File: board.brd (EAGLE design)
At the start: 53.3 x 41.9 mm, 6 parts, among them J1 POWER_JACK, J2 POWER_JACK, J3 POWER_JACK, J4 POWER_JACK, J5 POWER_JACK, J6 POWER_JACK

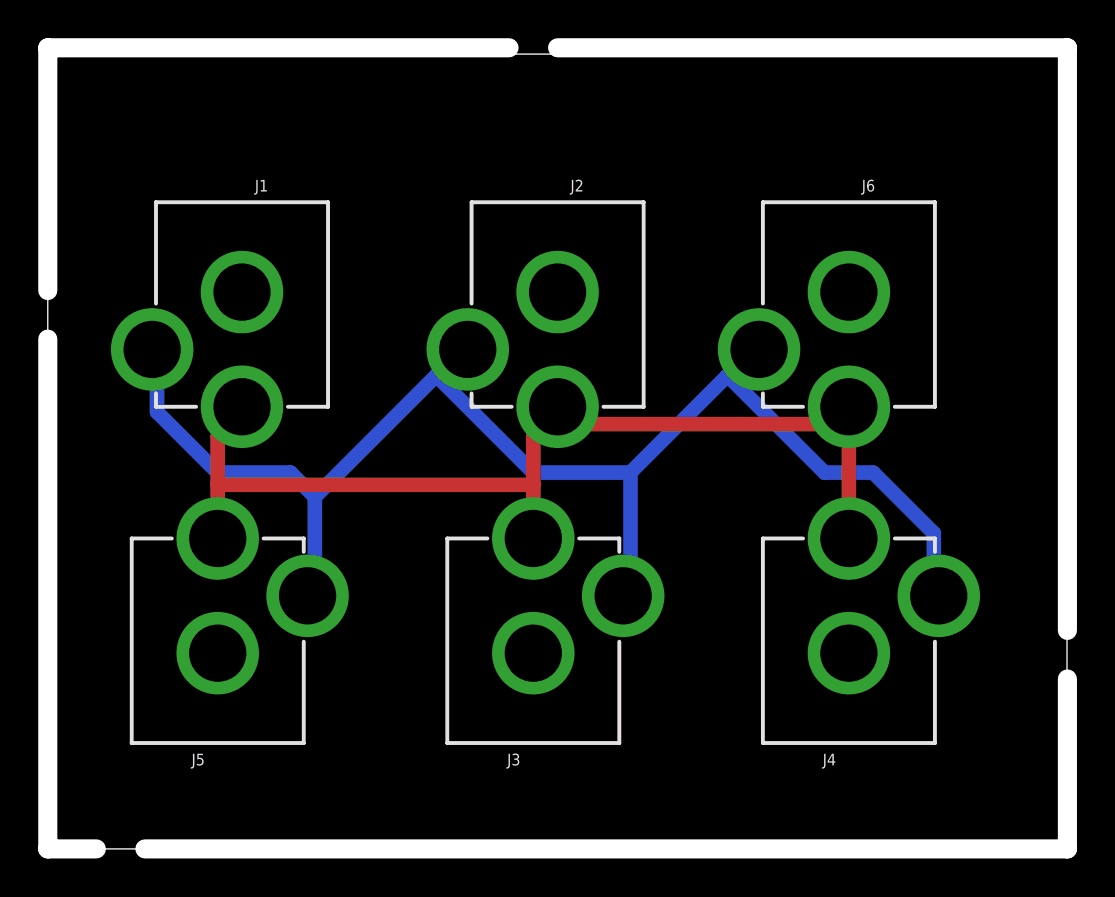
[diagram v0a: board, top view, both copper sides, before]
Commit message: git ignore, add cooper fills (for testing)
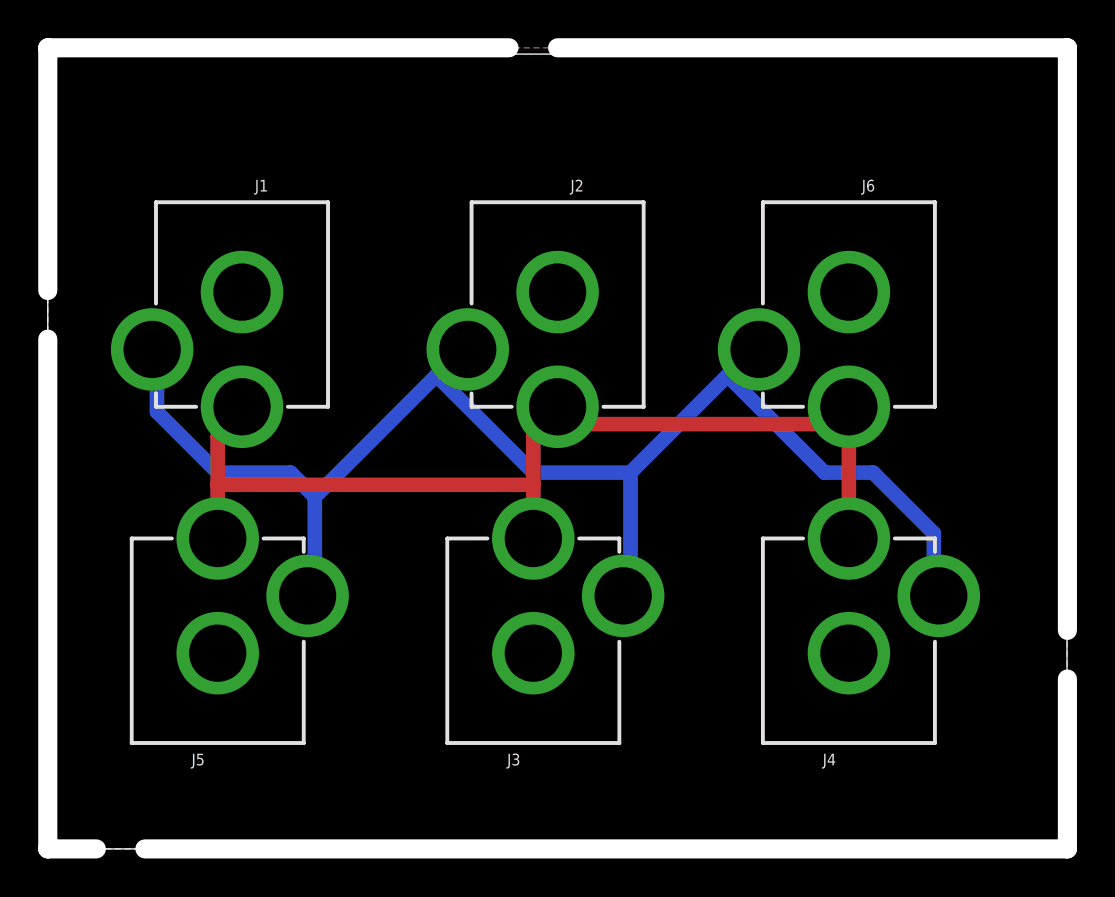
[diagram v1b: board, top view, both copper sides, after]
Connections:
- net N$1 renamed GND
- net N$2 renamed VCC
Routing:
- added copper zone on layer 1, net GND
- added copper zone on layer 16, net VCC
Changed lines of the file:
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@@
 </elements>
 <signals>
-<signal name="N$1">
-<contactref element="J1" pad="PWR"/>
-<contactref element="J5" pad="PWR"/>
-<contactref element="J4" pad="PWR"/>
-<contactref element="J3" pad="PWR"/>
-<contactref element="J2" pad="PWR"/>
-<contactref element="J6" pad="PWR"/>
-<wire x1="8.89" y1="21.59" x2="8.89" y2="19.05" width="0.762" layer="1"/>
-<wire x1="8.89" y1="19.05" x2="8.89" y2="16.24" width="0.762" layer="1"/>
-<wire x1="10.16" y1="22.86" x2="8.89" y2="21.59" width="0.762" layer="1"/>
-<wire x1="10.16" y1="22.86" x2="10.16" y2="23.13" width="0.762" layer="1"/>
-<wire x1="41.91" y1="23.13" x2="41.91" y2="22.225" width="0.762" layer="1"/>
-<wire x1="41.91" y1="22.225" x2="41.91" y2="16.24" width="0.762" layer="1"/>
-<wire x1="25.4" y1="21.59" x2="25.4" y2="19.05" width="0.762" layer="1"/>
-<wire x1="25.4" y1="19.05" x2="25.4" y2="16.24" width="0.762" layer="1"/>
-<wire x1="26.67" y1="22.86" x2="26.035" y2="22.225" width="0.762" layer="1"/>
-<wire x1="26.035" y1="22.225" x2="25.4" y2="21.59" width="0.762" layer="1"/>
-<wire x1="26.67" y1="22.86" x2="26.67" y2="23.13" width="0.762" layer="1"/>
-<wire x1="26.035" y1="22.225" x2="41.91" y2="22.225" width="0.762" layer="1"/>
-<wire x1="26.035" y1="22.225" x2="26.67" y2="23.13" width="0.762" layer="1"/>
-<wire x1="25.4" y1="19.05" x2="8.89" y2="19.05" width="0.762" layer="1"/>
-</signal>
-<signal name="N$2">
+<signal name="VCC">
 <contactref element="J1" pad="GNDBREAK"/>
 <contactref element="J5" pad="GNDBREAK"/>
@@
 <wire x1="30.48" y1="19.685" x2="25.4" y2="19.685" width="0.762" layer="16"/>
 <wire x1="20.32" y1="24.765" x2="21.97" y2="26.13" width="0.762" layer="16"/>
+<polygon width="0.1524" layer="16">
+<vertex x="0" y="41.91"/>
+<vertex x="0" y="0"/>
+<vertex x="53.34" y="0"/>
+<vertex x="53.34" y="41.91"/>
+</polygon>
+</signal>
+<signal name="GND">
+<polygon width="0.1524" layer="1">
+<vertex x="0" y="41.91"/>
+<vertex x="0" y="0"/>
+<vertex x="53.34" y="0"/>
+<vertex x="53.34" y="41.91"/>
+</polygon>
+<contactref element="J1" pad="PWR"/>
+<contactref element="J5" pad="PWR"/>
+<contactref element="J4" pad="PWR"/>
+<contactref element="J3" pad="PWR"/>
+<contactref element="J2" pad="PWR"/>
+<contactref element="J6" pad="PWR"/>
+<wire x1="8.89" y1="21.59" x2="8.89" y2="19.05" width="0.762" layer="1"/>
+<wire x1="8.89" y1="19.05" x2="8.89" y2="16.24" width="0.762" layer="1"/>
+<wire x1="10.16" y1="22.86" x2="8.89" y2="21.59" width="0.762" layer="1"/>
+<wire x1="10.16" y1="22.86" x2="10.16" y2="23.13" width="0.762" layer="1"/>
+<wire x1="41.91" y1="23.13" x2="41.91" y2="22.225" width="0.762" layer="1"/>
+<wire x1="41.91" y1="22.225" x2="41.91" y2="16.24" width="0.762" layer="1"/>
+<wire x1="25.4" y1="21.59" x2="25.4" y2="19.05" width="0.762" layer="1"/>
+<wire x1="25.4" y1="19.05" x2="25.4" y2="16.24" width="0.762" layer="1"/>
+<wire x1="26.67" y1="22.86" x2="26.035" y2="22.225" width="0.762" layer="1"/>
+<wire x1="26.035" y1="22.225" x2="25.4" y2="21.59" width="0.762" layer="1"/>
+<wire x1="26.67" y1="22.86" x2="26.67" y2="23.13" width="0.762" layer="1"/>
+<wire x1="26.035" y1="22.225" x2="41.91" y2="22.225" width="0.762" layer="1"/>
+<wire x1="26.035" y1="22.225" x2="26.67" y2="23.13" width="0.762" layer="1"/>
+<wire x1="25.4" y1="19.05" x2="8.89" y2="19.05" width="0.762" layer="1"/>
 </signal>
 </signals>
